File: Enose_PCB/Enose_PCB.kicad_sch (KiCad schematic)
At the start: 47 parts, among them IC3 TPS22958DGNR, J1 Conn_01x04_Pin, J10 Fan, J2 Conn_01x04_Pin, J3 Conn_01x04_Pin, J4 DA15_Pins, Q6 NMOS, SW1 SW_SPST, SW2 SW_SPST, SW4 SW_SPDT, U1 ESP32-S3-WROOM-1

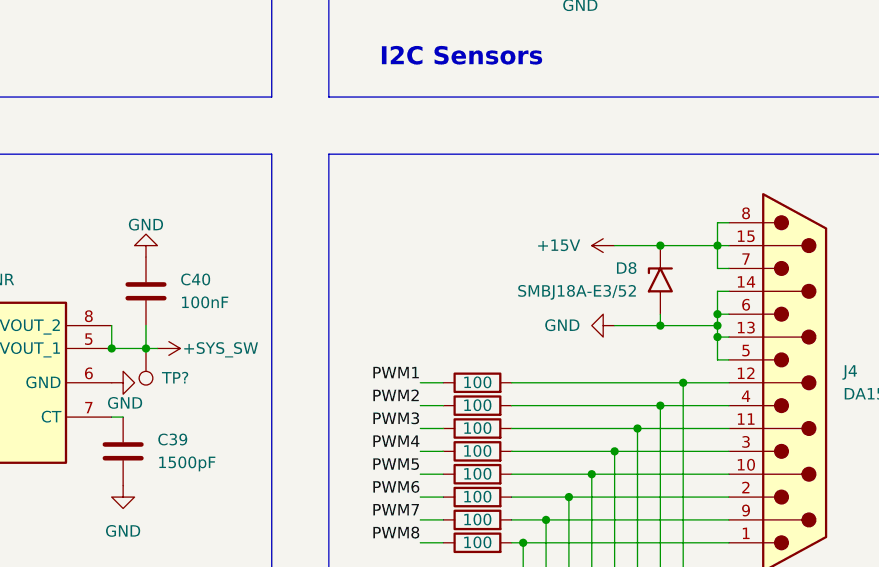
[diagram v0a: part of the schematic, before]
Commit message: Working on Enose PCB Layout
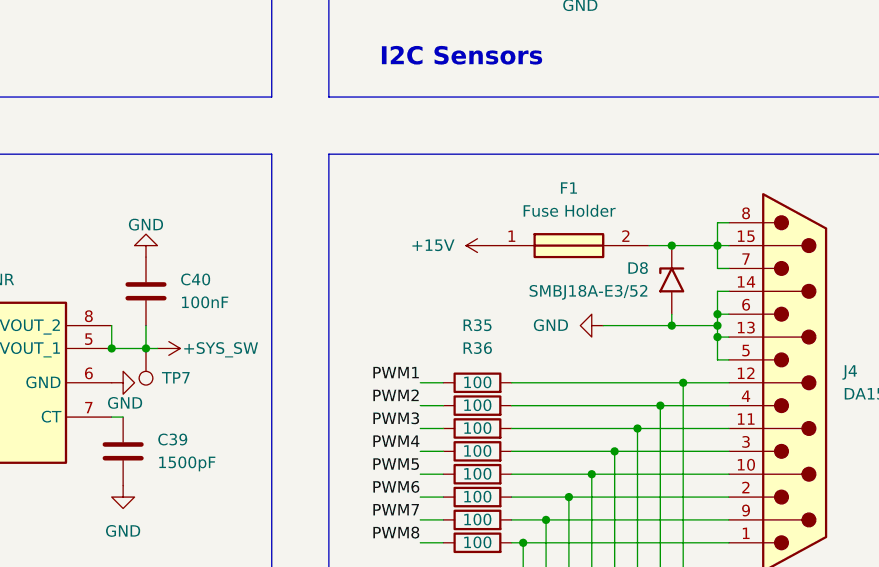
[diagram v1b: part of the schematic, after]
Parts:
- added F1: Fuse Holder, SamacSys_Parts:64600001223, symbol SamacSys_Parts:64600001223
- gave numbers to parts that had none: 1
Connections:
- net +15V: now also F1.1; no longer D8.1 (A1), J4.15 (P15), J4.7, J4.8
- new net: D8.1 (A1), F1.2, J4.15 (P15), J4.7, J4.8
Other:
- moved on the sheet: D8
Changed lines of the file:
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@@
 	)
 	(junction
+		(at 241.3 92.71)
+		(diameter 0)
+		(color 0 0 0 0)
+	)
+	(junction
 		(at 52.07 53.34)
 		(diameter 0)
@@
 	)
 	(junction
-		(at 240.03 92.71)
-		(diameter 0)
-		(color 0 0 0 0)
-	)
-	(junction
 		(at 67.31 43.18)
 		(diameter 0)
@@
 	)
 	(junction
-		(at 52.07 38.1)
+		(at 241.3 101.6)
 		(diameter 0)
 		(color 0 0 0 0)
 	)
 	(junction
-		(at 240.03 101.6)
+		(at 52.07 38.1)
 		(diameter 0)
 		(color 0 0 0 0)
@@
 	(wire
 		(pts
-			(xy 234.95 92.71) (xy 240.03 92.71)
+			(xy 223.52 54.61) (xy 231.14 54.61)
 		)
 		(stroke
@@
 	(wire
 		(pts
-			(xy 223.52 54.61) (xy 231.14 54.61)
+			(xy 48.26 93.98) (xy 52.07 93.98)
 		)
 		(stroke
@@
 	(wire
 		(pts
-			(xy 48.26 93.98) (xy 52.07 93.98)
+			(xy 181.61 48.26) (xy 181.61 46.99)
 		)
 		(stroke
@@
 	(wire
 		(pts
-			(xy 181.61 48.26) (xy 181.61 46.99)
+			(xy 38.1 135.89) (xy 38.1 138.43)
 		)
 		(stroke
@@
 	(wire
 		(pts
-			(xy 38.1 135.89) (xy 38.1 138.43)
+			(xy 238.76 92.71) (xy 241.3 92.71)
 		)
 		(stroke
@@
 	(wire
 		(pts
-			(xy 240.03 100.33) (xy 240.03 101.6)
-		)
-		(stroke
-			(width 0)
-			(type default)
-		)
-	)
-	(wire
-		(pts
 			(xy 143.51 104.14) (xy 143.51 107.95)
 		)
@@
 	(wire
 		(pts
+			(xy 241.3 92.71) (xy 246.38 92.71)
+		)
+		(stroke
+			(width 0)
+			(type default)
+		)
+	)
+	(wire
+		(pts
 			(xy 234.95 115.57) (xy 234.95 129.54)
 		)
@@
 	(wire
 		(pts
-			(xy 40.64 54.61) (xy 40.64 60.96)
+			(xy 241.3 100.33) (xy 241.3 101.6)
 		)
 		(stroke
@@
 	(wire
 		(pts
-			(xy 156.21 39.37) (xy 158.75 39.37)
+			(xy 40.64 54.61) (xy 40.64 60.96)
 		)
 		(stroke
@@
 	(wire
 		(pts
-			(xy 247.65 59.69) (xy 248.92 59.69)
+			(xy 156.21 39.37) (xy 158.75 39.37)
 		)
 		(stroke
@@
 	(wire
 		(pts
-			(xy 213.36 113.03) (xy 215.9 113.03)
+			(xy 247.65 59.69) (xy 248.92 59.69)
 		)
 		(stroke
@@
 	(wire
 		(pts
-			(xy 48.26 91.44) (xy 52.07 91.44)
+			(xy 213.36 113.03) (xy 215.9 113.03)
 		)
 		(stroke
@@
 	(wire
 		(pts
-			(xy 166.37 44.45) (xy 166.37 46.99)
+			(xy 48.26 91.44) (xy 52.07 91.44)
 		)
 		(stroke
@@
 	(wire
 		(pts
-			(xy 106.68 119.38) (xy 106.68 123.19)
+			(xy 166.37 44.45) (xy 166.37 46.99)
 		)
 		(stroke
@@
 	(wire
 		(pts
-			(xy 53.34 121.92) (xy 62.23 121.92)
+			(xy 106.68 119.38) (xy 106.68 123.19)
 		)
 		(stroke
@@
 	(wire
 		(pts
-			(xy 240.03 92.71) (xy 246.38 92.71)
+			(xy 53.34 121.92) (xy 62.23 121.92)
 		)
 		(stroke
@@
 	(wire
 		(pts
+			(xy 241.3 101.6) (xy 246.38 101.6)
+		)
+		(stroke
+			(width 0)
+			(type default)
+		)
+	)
+	(wire
+		(pts
 			(xy 48.26 76.2) (xy 52.07 76.2)
 		)
@@
 	(wire
 		(pts
-			(xy 234.95 101.6) (xy 240.03 101.6)
+			(xy 233.68 101.6) (xy 241.3 101.6)
 		)
 		(stroke
@@
 	(wire
 		(pts
-			(xy 240.03 101.6) (xy 246.38 101.6)
-		)
-		(stroke
-			(width 0)
-			(type default)
-		)
-	)
-	(wire
-		(pts
 			(xy 143.51 101.6) (xy 143.51 104.14)
 		)
@@
 	(symbol
 		(lib_id "power:GND")
-		(at 234.95 101.6 270)
+		(at 233.68 101.6 270)
 		(unit 1)
 		(exclude_from_sim no)
@@
 		(fields_autoplaced yes)
 		(property "Reference" "#PWR063"
-			(at 228.6 101.6 0)
+			(at 227.33 101.6 0)
 			(effects
 				(font
@@
 		)
 		(property "Value" "GND"
-			(at 231.14 101.5999 90)
+			(at 229.87 101.5999 90)
 			(effects
 				(font
@@
 		)
 		(property "Footprint" ""
-			(at 234.95 101.6 0)
+			(at 233.68 101.6 0)
 			(effects
 				(font
@@
 		)
 		(property "Datasheet" ""
-			(at 234.95 101.6 0)
+			(at 233.68 101.6 0)
 			(effects
 				(font
@@
 		)
 		(property "Description" "Power symbol creates a global label with name \"GND\" , ground"
-			(at 234.95 101.6 0)
+			(at 233.68 101.6 0)
 			(effects
 				(font
@@
 					(size 1.27 1.27)
 				)
-				(hide yes)
 			)
 		)
@@
 					(size 1.27 1.27)
 				)
-				(hide yes)
 			)
 		)
@@
 	)
 	(symbol
+		(lib_id "SamacSys_Parts:64600001223")
+		(at 220.98 92.71 0)
+		(unit 1)
+		(exclude_from_sim no)
+		(in_bom yes)
+		(on_board yes)
+		(dnp no)
+		(fields_autoplaced yes)
+		(property "Reference" "F1"
+			(at 229.87 86.36 0)
+			(effects
+				(font
+					(size 1.27 1.27)
+				)
+			)
+		)
+		(property "Value" "Fuse Holder"
+			(at 229.87 88.9 0)
+			(effects
+				(font
+					(size 1.27 1.27)
+				)
+			)
+		)
+		(property "Footprint" "SamacSys_Parts:64600001223"
+			(at 234.95 188.9 0)
+			(effects
+				(font
+					(size 1.27 1.27)
+				)
+				(justify left top)
+				(hide yes)
+			)
+		)
+		(property "Datasheet" "https://m.littelfuse.com/~/media/electronics/datasheets/fuse_blocks/littelfuse_fuse_block_646_datasheet.pdf.pdf"
+			(at 234.95 288.9 0)
+			(effects
+				(font
+					(size 1.27 1.27)
+				)
+				(justify left top)
+				(hide yes)
+			)
+		)
+		(property "Description" "LITTELFUSE - 64600001223 - FUSE BLOCK, 5X20MM, THROUGH HOLE"
+			(at 220.98 92.71 0)
+			(effects
+				(font
+					(size 1.27 1.27)
+				)
+				(hide yes)
+			)
+		)
+		(property "Height" "12"
+			(at 234.95 488.9 0)
+			(effects
+				(font
+					(size 1.27 1.27)
+				)
+				(justify left top)
+				(hide yes)
+			)
+		)
+		(property "Mouser Part Number" "576-64600001223"
+			(at 234.95 588.9 0)
+			(effects
+				(font
+					(size 1.27 1.27)
+				)
+				(justify left top)
+				(hide yes)
+			)
+		)
+		(property "Mouser Price/Stock" "https://www.mouser.co.uk/ProductDetail/Littelfuse/64600001223?qs=up76HT6PtJjfTS5uVso6wg%3D%3D"
+			(at 234.95 688.9 0)
+			(effects
+				(font
+					(size 1.27 1.27)
+				)
+				(justify left top)
+				(hide yes)
+			)
+		)
+		(property "Manufacturer_Name" "LITTELFUSE"
+			(at 234.95 788.9 0)
+			(effects
+				(font
+					(size 1.27 1.27)
+				)
+				(justify left top)
+				(hide yes)
+			)
+		)
+		(property "Manufacturer_Part_Number" "64600001223"
+			(at 234.95 888.9 0)
+			(effects
+				(font
+					(size 1.27 1.27)
+				)
+				(justify left top)
+				(hide yes)
+			)
+		)
+		(pin "1"
+		)
+		(pin "2"
+		)
+		(instances
+			(project ""
+				(path "/eef70be0-4107-491c-8ca0-465071a6397e"
+					(reference "F1")
+					(unit 1)
+				)
+			)
+		)
+	)
+	(symbol
 		(lib_id "Device:C")
 		(at 231.14 58.42 0)
@@
 	(symbol
 		(lib_id "power:+15V")
-		(at 234.95 92.71 90)
+		(at 220.98 92.71 90)
 		(unit 1)
 		(exclude_from_sim no)
@@
 		(fields_autoplaced yes)
 		(property "Reference" "#PWR062"
-			(at 238.76 92.71 0)
+			(at 224.79 92.71 0)
 			(effects
 				(font
@@
 		)
 		(property "Value" "+15V"
-			(at 231.14 92.7099 90)
+			(at 217.17 92.7099 90)
 			(effects
 				(font
@@
 		)
 		(property "Footprint" ""
-			(at 234.95 92.71 0)
+			(at 220.98 92.71 0)
 			(effects
 				(font
@@
 		)
 		(property "Datasheet" ""
-			(at 234.95 92.71 0)
+			(at 220.98 92.71 0)
 			(effects
 				(font
@@
 		)
 		(property "Description" "Power symbol creates a global label with name \"+15V\""
-			(at 234.95 92.71 0)
+			(at 220.98 92.71 0)
 			(effects
 				(font
@@
 	(symbol
 		(lib_id "Diode:SM6T18A")
-		(at 240.03 96.52 90)
+		(at 241.3 96.52 90)
 		(mirror x)
 		(unit 1)
@@
 		(dnp no)
 		(property "Reference" "D8"
-			(at 237.49 95.2499 90)
+			(at 238.76 95.2499 90)
 			(effects
 				(font
@@
 		)
 		(property "Value" "SMBJ18A-E3/52"
-			(at 237.49 97.7899 90)
+			(at 238.76 97.7899 90)
 			(effects
 				(font
@@
 		)
 		(property "Footprint" "Diode_SMD:D_SMB"
-			(at 245.11 96.52 0)
+			(at 246.38 96.52 0)
 			(effects
 				(font
@@
 		)
 		(property "Datasheet" "http://www.vishay.com/docs/88392/smbj.pdf"
-			(at 240.03 95.25 0)
+			(at 241.3 95.25 0)
 			(effects
 				(font
@@
 		)
 		(property "Description" "Vishay SMBJ18A-E3/52, Uni-Directional TVS Diode, 600W, 2-Pin DO-214AA"
-			(at 240.03 96.52 0)
+			(at 241.3 96.52 0)
 			(effects
 				(font
@@
 		(on_board yes)
 		(dnp no)
-		(property "Reference" "TP?"
+		(property "Reference" "TP7"
 			(at 184.658 107.442 0)
 			(effects
@@
 			(project "Enose_PCB"
 				(path "/eef70be0-4107-491c-8ca0-465071a6397e"
-					(reference "TP?")
+					(reference "TP7")
 					(unit 1)
 				)
